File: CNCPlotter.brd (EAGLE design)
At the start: 172.4 x 76.8 mm, 125 parts, among them IC1 HEF4050B, IC2 MC34063, IC3 LD1117S33, IC4 74HC4094, IC5 ATmega32U4, IC6 DRV8811, IC7 DRV8811, J1 Home Switches, J10 ISP, J11 X Motor, J12 MS1, J13 MS0, J14 Y Motor, J15 MS1, J16 MS0, J2 Touchscreen, J3 12V Supply, J4 MicroSD Card, J5 HWB, J6 USB-FT, J7 Servo, J8 Z Drive, J9 UART, Q1 16MHz

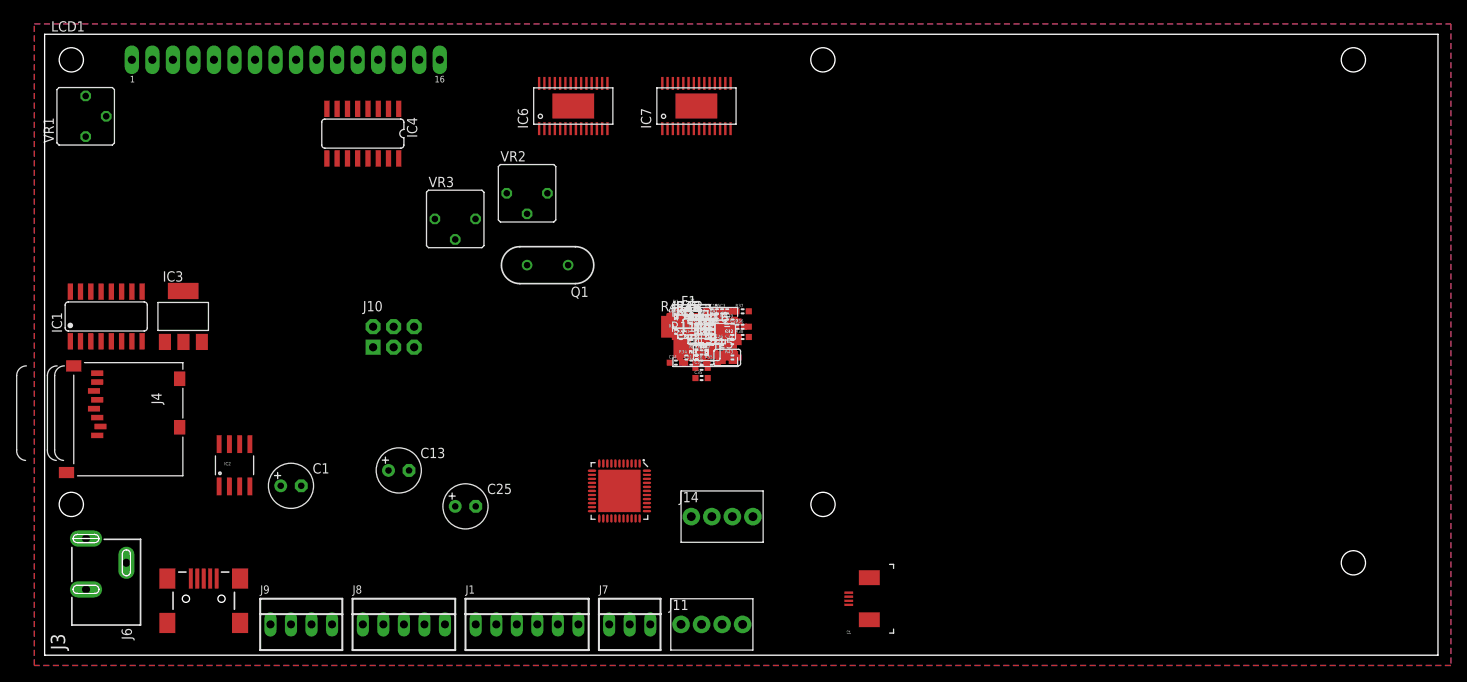
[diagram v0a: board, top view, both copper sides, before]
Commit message: foo
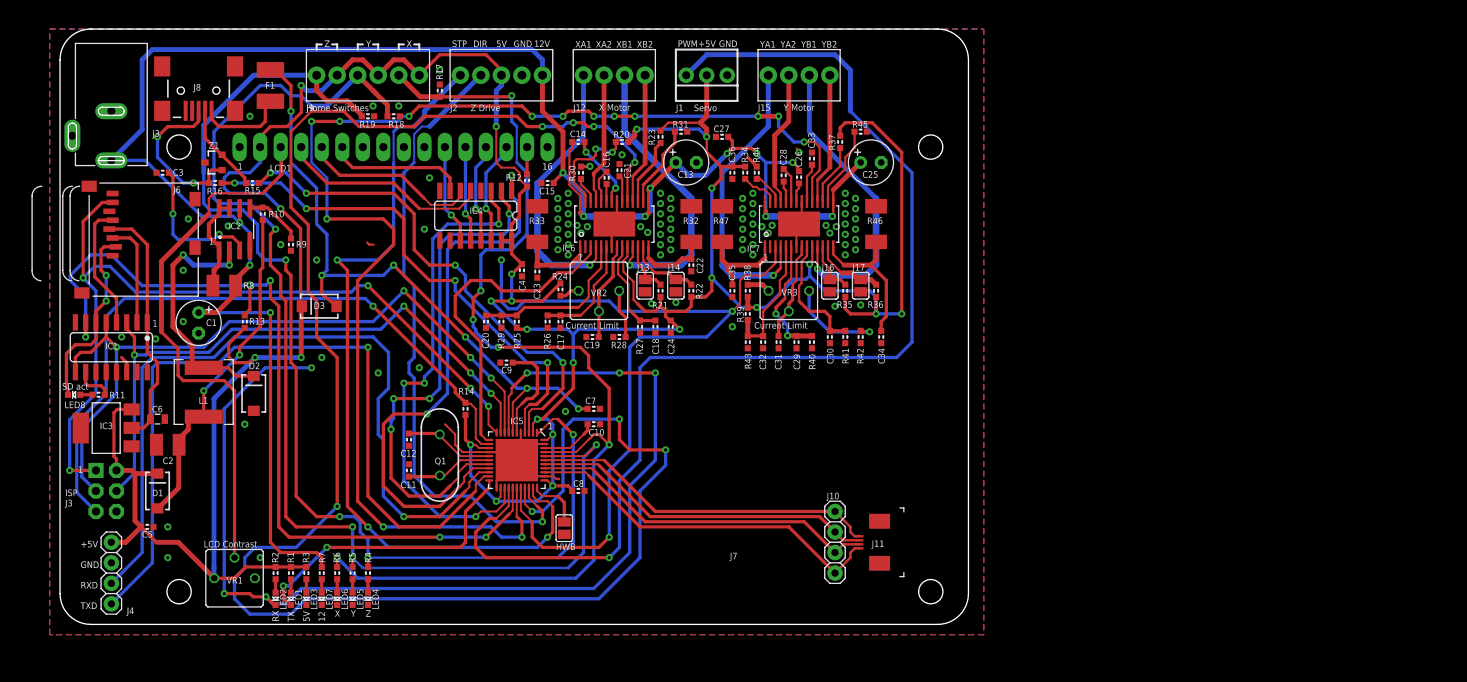
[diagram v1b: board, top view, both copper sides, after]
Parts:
- added J17: MS0, freetronics-luke:SJ
- C1, C13, C25: value 100 uF -> 100uF
- C10, C7, C8: value 100nF -> 100 nF; device freetronics:0603 -> freetronics-master-v1:0603
- C11, C12: device freetronics:0603 -> freetronics-master-v1:0603
- C17, C18, C29, C30: value 680 pF -> 1nF
- C9: value 1uF -> 1 uF; device freetronics:0603 -> freetronics-master-v1:0603
- F1: value 500mA PPTC -> 500mA
- J1: value Home Switches -> Servo; device con-molex:22-23-2061 -> con-molex:22-23-2031
- J10: value ISP -> Touchscreen; device SparkFun:2X3-NS -> pinhead:1X04
- J11: value X Motor -> Touchscreen; device con-phoenix-254:4POL254 -> SparkFun:DS_TOUCH_CONNECTOR
- J12: value MS1 -> X Motor; device freetronics-luke:SJ -> con-phoenix-254:4POL254
- J13, J16: value MS0 -> MS1
- J14: value Y Motor -> MS0; device con-phoenix-254:4POL254 -> freetronics-luke:SJ
- J15: value MS1 -> Y Motor; device freetronics-luke:SJ -> con-phoenix-254:4POL254
- J2: value Touchscreen -> Z Drive; device SparkFun:DS_TOUCH_CONNECTOR -> con-phoenix-254:5POL254
- J3: value 12V Supply -> ISP; device SparkFun:POWER_JACK_SLOT -> SparkFun:2X3-NS
- J4: value MicroSD Card -> UART; device RAMPSdisplay:ADAFRUIT_MICROSD -> pinhead:1X04
- J5: value HWB -> 12V Supply; device freetronics-luke:SJ -> SparkFun:POWER_JACK_SLOT
- J6: value USB-FT -> MicroSD Card; device freetronics-luke:USB-MINIB-FT -> RAMPSdisplay:ADAFRUIT_MICROSD
- J7: value Servo -> HWB; device con-molex:22-23-2031 -> freetronics-luke:SJ
- J8: value Z Drive -> USB-FT; device con-molex:22-23-2051 -> freetronics-luke:USB-MINIB-FT
- J9: value UART -> Home Switches; device con-molex:22-23-2041 -> con-phoenix-254:6POL254
- LED1: value TXD -> TX
- LED2: value RXD -> RX
- LED4: value Z Home -> Z
- LED5: value Y Home -> Y
- LED6: value X Home -> X
- LED7: value 12V -> 12
- R10: value 10k -> 3k0
- R11: value 0.2 ohms -> 1k; device rcl:R1210 -> freetronics-master-v1:0603
- R12: value 1k -> 22R
- R13: value 3k0 -> 10k
- R14: value 1k -> 10k
- R16: value 10k -> 22R
- R18, R19: value 22R -> 10k
- R20, R21, R22, R23, R25, R30, R31: value 10k -> 10K
- R24: value 3k3 -> 3K3
- R26, R27, R40, R41: value 56k -> 47K
- R29, R43: value 4k7 -> 4K7
- R32, R33: value 0.2R 1W -> 0.25R 1W
- R8: value 10k -> 0.2 ohms; device freetronics-master-v1:0603 -> rcl:R1210
- R9: value 10k -> 1k
- VR2: value 10 k -> 10K
- moved J2 79.3 mm to (54.6, 67.9), turned to 180 degrees
- moved J5 78.6 mm to (6.35, 63.5), turned to 180 degrees
- moved LED8 78.2 mm to (1.75, 28.4), turned to 180 degrees
- moved R11 73.6 mm to (4.76, 28.4)
- moved J8 71.9 mm to (17.1, 67.3), turned to 270 degrees
- moved C3 71.9 mm to (12.7, 55.9), turned to 180 degrees
- moved C6 71.5 mm to (12.1, 25.4)
- moved J1 71.5 mm to (80.0, 67.9), turned to 180 degrees
- moved C5 70.4 mm to (10.8, 12.1)
- moved D1 69.5 mm to (12.1, 16.5), turned to 90 degrees
- moved J9 68.4 mm to (38.1, 67.9), turned to 180 degrees
- moved C2 67.6 mm to (13.3, 22.2), turned to 180 degrees
- moved C25 65.8 mm to (100.3, 57.1)
- moved R16 63.3 mm to (19.2, 54.6), turned to 180 degrees
- moved Z1 62.7 mm to (19.1, 57.1), turned to 90 degrees
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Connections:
- new net N$71: R42.2, VR3.A
- net !RESET: now also J3.5, R14.1; no longer J10.5, R17.1
- net !SD_CS: now also R13.1; no longer R16.1
- net +12V: now also J2.1, J5.PWR, R8.1; no longer J3.PWR, J8.1, R11.1
- net +5V: now also J1.2, J2.3, J3.2, J4.1, J9.3, J9.5, R12.2, R13.2, R14.2; no longer J1.1, J1.3, J1.5, J10.2, J7.2, J8.3, R15.2, R16.2, R17.2
- net FOO: now also J6.2; no longer J4.2
- net GND: now also C7.2, J1.1, J14.1, J17.1, J2.2, J3.6, J4.2, J5.GND, J6.6, J6.MT1, J6.MT2, J8.GND, J8.SH1, J8.SH2, J8.SH3, J8.SH4, R17.2, R18.2, R19.2; no longer C7.1, J10.6, J12.1, J15.1, J3.GND@1, J4.6, J4.MT1, J4.MT2, J5.1, J6.GND, J6.SH1, J6.SH2, J6.SH3, J6.SH4, J8.2, J9.2, R10.2, R12.2, R8.2
- net HWB: now also J7.2; no longer J5.2
- net MISO: now also J3.1, J6.7; no longer J10.1, J4.7
- net MOSI: now also J3.4; no longer J10.4
- net MOSI_3.3V: now also J6.3; no longer J4.3
- net N$1: now also J15.1; no longer J14.1
- net N$2: now also J8.VBUS; no longer J6.VBUS
- net N$20: no longer R42.2, VR3.A
- net N$21: now also J12.4; no longer J11.4
- net N$22: now also J12.3; no longer J11.3
- net N$23: now also J12.2; no longer J11.2
- net N$3: now also J12.1; no longer J11.1
- net N$32: now also R8.2; no longer R11.2
- net N$33: now also J8.D+, R16.2; no longer J6.D+, R19.2
- net N$34: now also J8.D-, R15.2; no longer J6.D-, R18.2
- net N$37: now also R16.1; no longer R19.1
- net N$38: now also R15.1; no longer R18.1
- net N$4: now also J15.4; no longer J14.4
- net N$40: now also C7.1; no longer C7.2
- net N$44: now also R10.2, R9.1; no longer R12.1, R13.2
- net N$5: now also J15.3; no longer J14.3
- net N$59: now also R12.1; no longer R15.1
- net N$6: now also J15.2; no longer J14.2
- net N$62: now also R11.1; no longer R14.1
- net N$63: now also R11.2; no longer R14.2
- net N$66: now also J13.2; no longer J12.2
- net N$67: now also J14.2; no longer J13.2
- net N$74: now also J16.2; no longer J15.2
- net N$75: now also J17.2; no longer J16.2
- net REG_5V: now also R10.1; no longer R13.1
- net RXD: now also J4.3; no longer J9.3
- net SCK: now also J3.3; no longer J10.3
- net SCK_3.3V: now also J6.5; no longer J4.5
- net SERVO: now also J1.3; no longer J7.3
- net TOUCH1: now also J10.1, J11.Y1; no longer J2.Y1
- net TOUCH2: now also J10.2, J11.X2; no longer J2.X2
- net TOUCH3: now also J10.3, J11.Y2; no longer J2.Y2
- net TOUCH4: now also J10.4, J11.X1; no longer J2.X1
- net TXD: now also J4.4; no longer J9.4
- net VDD: now also J6.4; no longer J4.4
- net X_HOME: now also J9.2, R17.1; no longer J1.2, R8.1
- net Y_HOME: now also J9.4, R18.1; no longer J1.4, R9.1
- net Z_DIR: now also J2.4; no longer J8.4
- net Z_HOME: now also J9.6, R19.1; no longer J1.6, R10.1
- net Z_STEP: now also J2.5; no longer J8.5
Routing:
- net +5V: track 0.00 -> 445.8 mm, vias 0 -> 24
- net +12V: track 0.00 -> 244.9 mm, vias 0 -> 12
- net X_STEP: track 0.00 -> 222.4 mm, vias 0 -> 8
- net Y_STEP: track 0.00 -> 159.8 mm, vias 0 -> 14
- net Z_HOME: track 0.00 -> 149.3 mm, vias 0 -> 4
- net Y_HOME: track 0.00 -> 148.2 mm, vias 0 -> 4
- net SERVO: track 0.00 -> 145.6 mm, vias 0 -> 1
- net RXLED: track 0.00 -> 138.4 mm, vias 0 -> 6
- net X_HOME: track 0.00 -> 136.9 mm, vias 0 -> 6
- net !SD_CS: track 0.00 -> 106.9 mm, vias 0 -> 5
- net MISO: track 0.00 -> 102.9 mm, vias 0 -> 5
- net Y_DIR: track 0.00 -> 102.9 mm, vias 0 -> 3
- net Z_STEP: track 0.00 -> 101.7 mm, vias 0 -> 3
- net TXD: track 0.00 -> 97.1 mm, vias 0 -> 1
- net RXD: track 0.00 -> 96.5 mm, vias 0 -> 1
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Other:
- board size 172.4 x 76.8 mm -> 112.4 x 73.7 mm
- board text added: "+5V"
- board text added: "1"
- board text added: "12V"
- board text added: "5V"
- board text added: "Current Limit"
- board text added: "DIR"
- board text added: "GND"
- board text added: "HWB"
- board text added: "Home Switches"
- board text added: "IC5"
- board text added: "J3"
- board text added: "L1"
- board text added: "LCD Contrast"
- board text added: "PWM"
- board text added: "RXD"
- board text added: "STP"
- board text added: "TXD"
- board text added: "X"
- board text added: "XA1"
- board text added: "XA2"
- board text added: "XB1"
- board text added: "XB2"
- board text added: "Y"
- board text added: "YA1"
- board text added: "YA2"
- board text added: "YB1"
- board text added: "YB2"
- board text added: "Z"

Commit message: foo
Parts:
- R32, R33: value 0.25R 1W -> 0.20Ω 1W
- R46, R47: value 0.2R 1W -> 0.20Ω 1W
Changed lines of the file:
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@@
 <attribute name="VALUE" x="81.1784" y="6.223" size="0.8128" layer="27" ratio="15"/>
 </element>
-<element name="R32" library="rcl" package="R2010" value="0.25R 1W" x="78.105" y="49.53" smashed="yes" rot="R270">
+<element name="R32" library="rcl" package="R2010" value="0.20Ω 1W" x="78.105" y="49.53" smashed="yes" rot="R270">
 <attribute name="NAME" x="77.073125" y="49.53" size="0.8128" layer="25" ratio="15"/>
 <attribute name="VALUE" x="79.375" y="7.62" size="0.8128" layer="27" ratio="15"/>
@@
 <attribute name="VALUE" x="82.804" y="8.8773" size="0.8128" layer="27" font="vector" ratio="15"/>
 </element>
-<element name="R33" library="rcl" package="R2010" value="0.25R 1W" x="59.055" y="49.53" smashed="yes" rot="R270">
+<element name="R33" library="rcl" package="R2010" value="0.20Ω 1W" x="59.055" y="49.53" smashed="yes" rot="R270">
 <attribute name="NAME" x="58.023125" y="49.53" size="0.8128" layer="25" ratio="15"/>
 <attribute name="VALUE" x="78.105" y="7.62" size="0.8128" layer="27" ratio="15"/>
@@
 <attribute name="VALUE" x="78.0034" y="5.588" size="0.8128" layer="27" ratio="15"/>
 </element>
-<element name="R46" library="rcl" package="R2010" value="0.2R 1W" x="100.965" y="49.53" smashed="yes" rot="R270">
+<element name="R46" library="rcl" package="R2010" value="0.20Ω 1W" x="100.965" y="49.53" smashed="yes" rot="R270">
 <attribute name="NAME" x="99.85375" y="49.53" size="0.8128" layer="25" ratio="15"/>
 <attribute name="VALUE" x="79.21625" y="6.19125" size="0.8128" layer="27" ratio="15"/>
@@
 <attribute name="VALUE" x="79.3115" y="6.6548" size="0.8128" layer="27" font="vector" ratio="15"/>
 </element>
-<element name="R47" library="rcl" package="R2010" value="0.2R 1W" x="81.915" y="49.53" smashed="yes" rot="R270">
+<element name="R47" library="rcl" package="R2010" value="0.20Ω 1W" x="81.915" y="49.53" smashed="yes" rot="R270">
 <attribute name="NAME" x="80.80375" y="49.53" size="0.8128" layer="25" ratio="15"/>
 <attribute name="VALUE" x="78.74" y="6.985" size="0.8128" layer="27" ratio="15"/>
@@
 </signal>
 </signals>
-<errors>
-</errors>
 </board>
 </drawing>
